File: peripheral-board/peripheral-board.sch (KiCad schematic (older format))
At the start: 12 parts, among them CON1001 AVR-ISP-10, P1001 Peripheral Bus, P1002 Power, SW1001 Power, U1001 ATTINY48-A

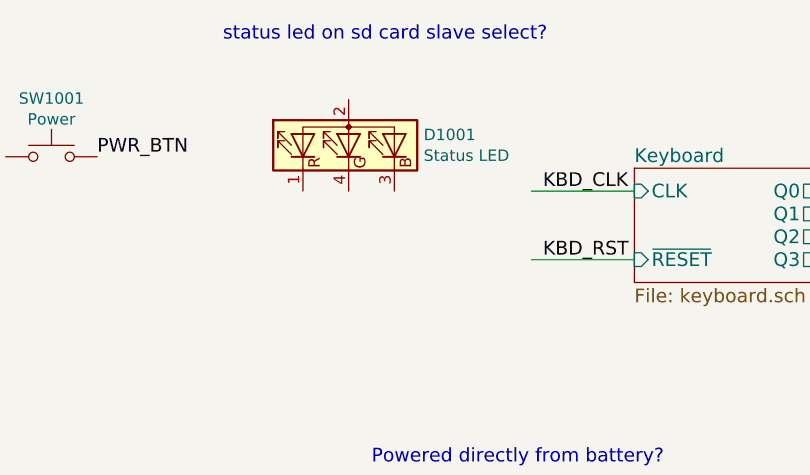
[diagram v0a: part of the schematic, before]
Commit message: routed spi
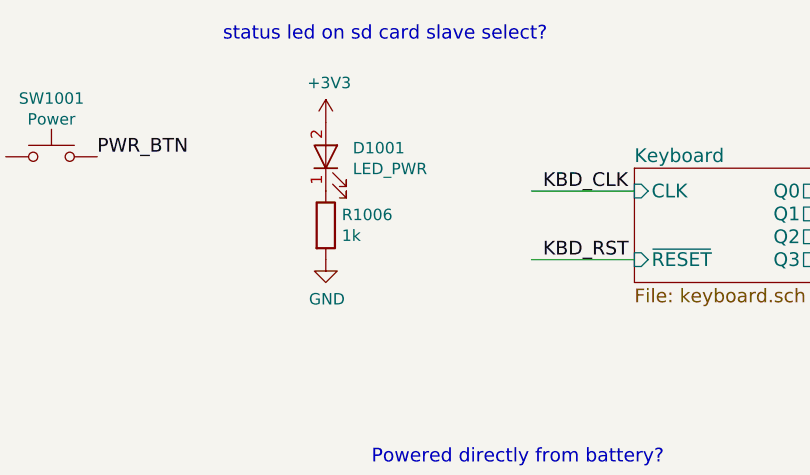
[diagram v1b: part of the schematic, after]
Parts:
- removed D1001: Status LED, symbol LED_RABG
- added D1001: LED_PWR, LEDs:LED-3MM, symbol LED
- added R1006: 1k, Resistors_SMD:R_0805, symbol R
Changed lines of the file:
@@
 	1    0    0    -1
-$EndComp
-$Comp
-L LED_RABG D1001
-U 1 1 582399DC
-P 3350 1250
-F 0 "D1001" V 3396 922 50  0000 R CNN
-F 1 "Status LED" V 3305 922 50  0000 R CNN
-F 2 "" H 3300 1200 50  0001 C CNN
-F 3 "" H 3300 1200 50  0000 C CNN
-	1    3350 1250
-	0    -1   -1   0
 $EndComp
 Text Notes 2800 800  0    60   ~ 0
@@
 Wire Wire Line
 	4950 3950 5450 3950
+$Comp
+L LED D1001
+U 1 1 58A4D1EF
+P 3250 1300
+F 0 "D1001" V 3288 1182 50  0000 R CNN
+F 1 "LED_PWR" V 3197 1182 50  0000 R CNN
+F 2 "LEDs:LED-3MM" H -50 -750 50  0001 C CNN
+F 3 "" H -50 -750 50  0001 C CNN
+	1    3250 1300
+	0    -1   -1   0
+$EndComp
+$Comp
+L R R1006
+U 1 1 58A4D893
+P 3250 1600
+F 0 "R1006" H 3320 1646 50  0000 L CNN
+F 1 "1k" H 3320 1555 50  0000 L CNN
+F 2 "Resistors_SMD:R_0805" V -170 -400 50  0001 C CNN
+F 3 "" H -100 -400 50  0001 C CNN
+	1    3250 1600
+	1    0    0    -1
+$EndComp
+$Comp
+L GND #PWR015
+U 1 1 58A4D9DD
+P 3250 1750
+F 0 "#PWR015" H -50 -250 50  0001 C CNN
+F 1 "GND" H 3255 1577 50  0000 C CNN
+F 2 "" H -50 0   50  0001 C CNN
+F 3 "" H -50 0   50  0001 C CNN
+	1    3250 1750
+	1    0    0    -1
+$EndComp
+$Comp
+L +3V3 #PWR016
+U 1 1 58A4DB27
+P 3250 1150
+F 0 "#PWR016" H -200 -800 50  0001 C CNN
+F 1 "+3V3" H 3265 1323 50  0000 C CNN
+F 2 "" H -200 -650 50  0001 C CNN
+F 3 "" H -200 -650 50  0001 C CNN
+	1    3250 1150
+	1    0    0    -1
+$EndComp
 $EndSCHEMATC
